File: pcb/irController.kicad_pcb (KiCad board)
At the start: 2 copper layers, 49 x 34 mm, 33 parts, among them J1 B4B-PH-K-S(LF)(SN), P1 ZX62R-B-5P, P2 GPIO_USER, Q1 Q_NMOS, SW2 SKRPACE010, U1 NJM2845, U2 ESP-13-WROOM-02, U3 IRSNS_GP1UXC41QS

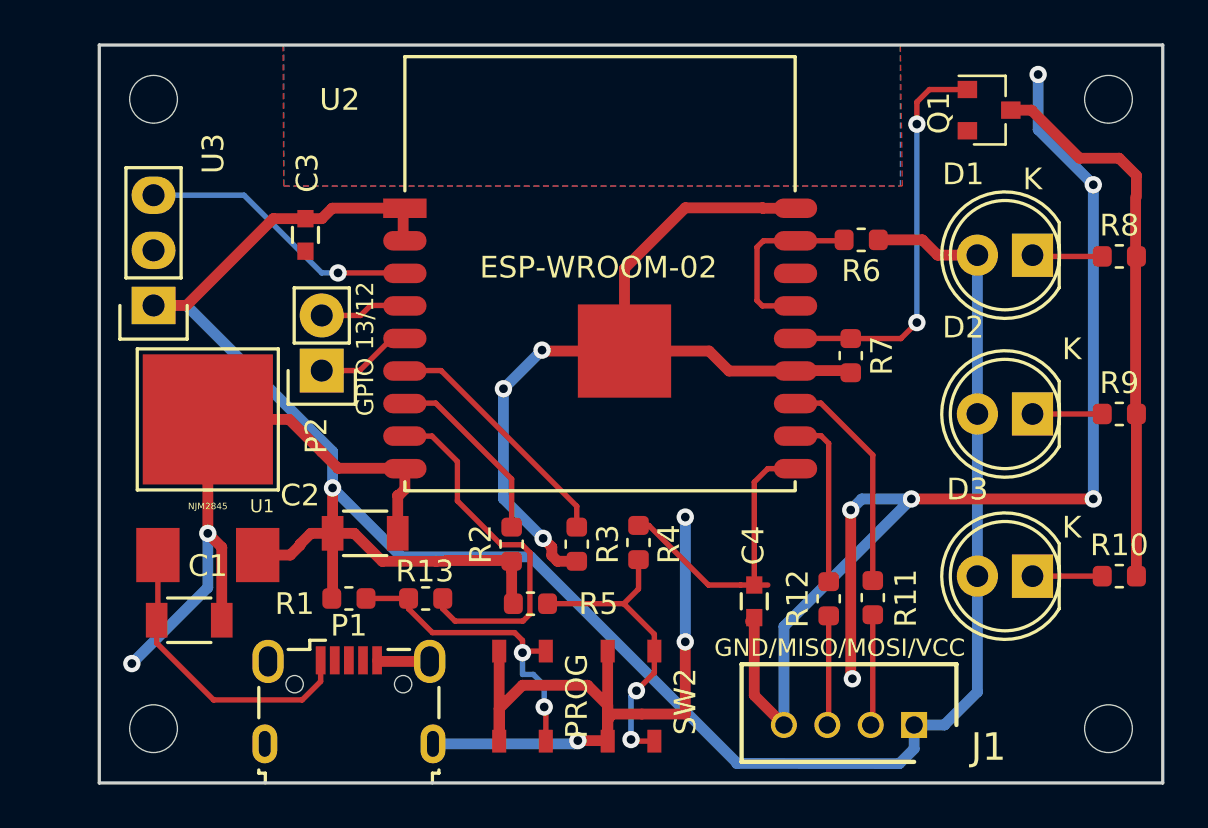
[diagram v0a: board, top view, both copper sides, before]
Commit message: パターン引いた
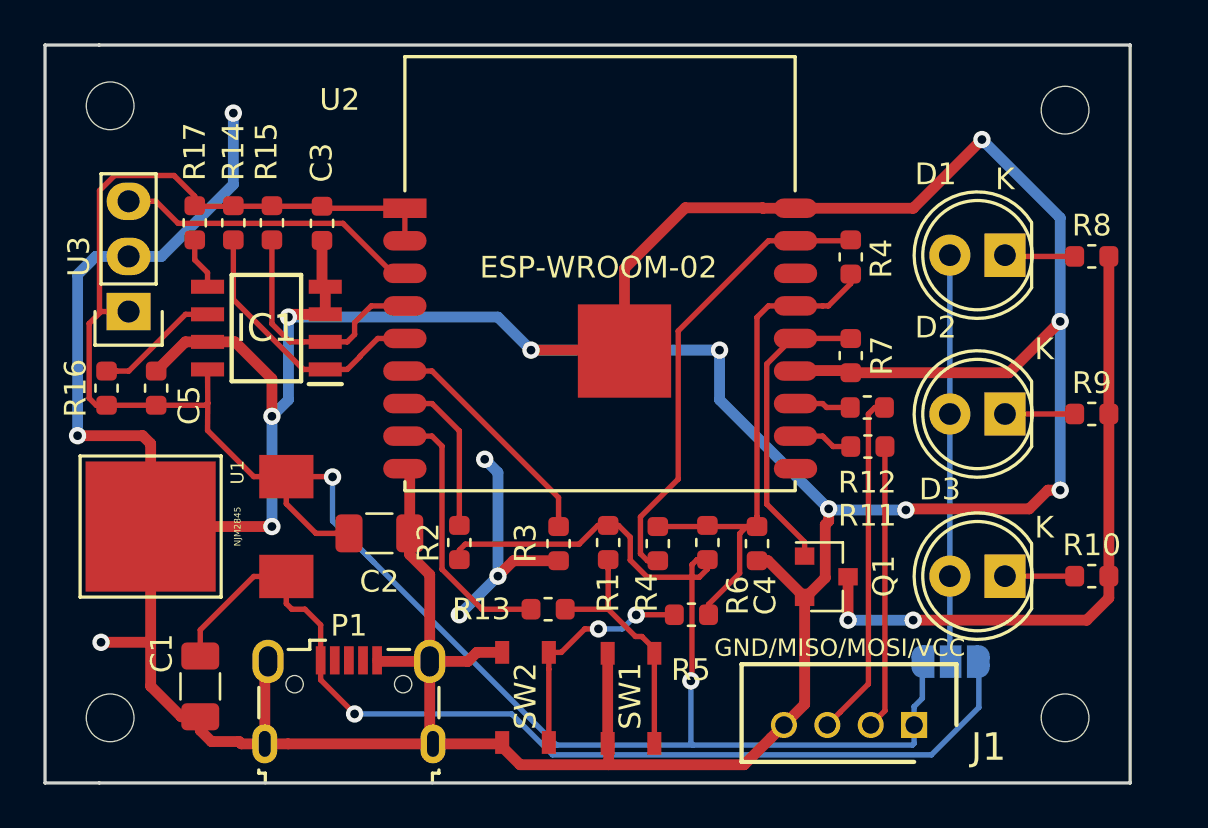
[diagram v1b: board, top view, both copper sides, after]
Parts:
- removed the ? at (134.5, 71.5)
- removed the ? at (134.5, 100.5)
- removed P2: GPIO_USER, Socket_Strips:Socket_Strip_Straight_1x02
- removed PROG: SKRPACE010, OriginalLibSw:SKRPACE010
- added ?: MountingHole_2.2mm_M2, Mounting_Holes:MountingHole_2.2mm_M2, F.Cu at (132.5, 71.8)
- added ?: MountingHole_2.2mm_M2, Mounting_Holes:MountingHole_2.2mm_M2, F.Cu at (132.5, 100.0)
- added C5: 0.1u, Capacitor_SMD:C_0603_1608Metric, F.Cu at (134.6, 84.8)
- added IC1: ADT7410TRZ, SamacSys:SOIC127P600X175-8N, F.Cu at (139.7, 82.0)
- added JP1: SolderJumper_3_Open, Jumper:SolderJumper-3_P1.3mm_Open_RoundedPad1.0x1.5mm_NumberLabels, B.Cu at (171.2, 97.4)
- added R14: 10k, Resistor_SMD:R_0603_1608Metric, F.Cu at (138.2, 77.2)
- added R15: 10k, Resistor_SMD:R_0603_1608Metric, F.Cu at (140.0, 77.2)
- added R16: 10k, Resistor_SMD:R_0603_1608Metric, F.Cu at (132.3, 84.8)
- added R17: 10k, Resistor_SMD:R_0603_1608Metric, F.Cu at (136.4, 77.2)
- added R4: 1k, Resistor_SMD:R_0603_1608Metric, F.Cu at (157.7, 92.0)
- added SW1: SKRPACE010, OriginalLibSw:SKRPACE010, F.Cu at (156.5, 99.1)
- C1, C2: footprint Capacitors_SMD:C_1206 -> Capacitor_SMD:C_1206_3216Metric
- C3: value 0.22u -> 0.1u; footprint Capacitors_SMD:C_0603 -> Capacitor_SMD:C_0603_1608Metric
- C4: footprint Capacitors_SMD:C_0603 -> Capacitor_SMD:C_0603_1608Metric
- R4, R5: value 10k -> 1k
- moved Q1 22.8 mm to (165.5, 93.5)
- moved R4 16.4 mm to (166.6, 78.8)
- moved R6 15.6 mm to (160.0, 91.9), turned to 90 degrees
- moved R1 12.2 mm to (155.4, 91.9), turned to 270 degrees
- moved R12 8.99 mm to (167.4, 85.7), turned to 180 degrees
- moved R5 7.43 mm to (159.3, 95.2), turned to 180 degrees
- moved R11 6.97 mm to (167.4, 87.5), turned to 180 degrees
- moved R13 5.66 mm to (152.7, 95.0), turned to 0 degrees
- moved U1 5.59 mm to (134.4, 91.2), turned to 90 degrees
- moved SW2 4.86 mm to (151.6, 99.1)
- moved C1 3.09 mm to (136.7, 98.6), turned to 270 degrees
- moved C4 2.66 mm to (162.3, 92.0)
- moved R2 2.41 mm to (148.6, 91.9)
- moved ? 2.06 mm to (176.5, 100.0)
- moved ? 2.06 mm to (176.5, 72.0)
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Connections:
- net Net-(C1-Pad1) renamed +5V
- C2 pad 1: Net-(C2-Pad1) -> +3V3
- C3 pad 1: Net-(C2-Pad1) -> +3V3
- D1 pad 2: Net-(C2-Pad1) -> Net-(D1-Pad2)
- D2 pad 2: Net-(C2-Pad1) -> Net-(D1-Pad2)
- D3 pad 2: Net-(C2-Pad1) -> Net-(D1-Pad2)
- J1 pad 1: Net-(C2-Pad1) -> +3V3
- R1 pad 1: Net-(C2-Pad1) -> +3V3
- R2 pad 1: Net-(C2-Pad1) -> +3V3
- R4 pad 1: Net-(R4-Pad1) -> Net-(C4-Pad1)
- R4 pad 2: Net-(C4-Pad1) -> Net-(R4-Pad2)
- R5 pad 1: Net-(C2-Pad1) -> Net-(C4-Pad1)
- R5 pad 2: Net-(R4-Pad1) -> Net-(R5-Pad2)
- R6 pad 1: Net-(C2-Pad1) -> +3V3
- R6 pad 2: Net-(R6-Pad2) -> Net-(C4-Pad1)
- SW2 pad 1: Net-(R4-Pad1) -> Net-(R5-Pad2)
- SW2 pad 3: Net-(R4-Pad1) -> Net-(R5-Pad2)
- U1 pad VO: Net-(C2-Pad1) -> +3V3
- U2 pad 1: Net-(C2-Pad1) -> +3V3
- U2 pad 10: Net-(C4-Pad1) -> Net-(U2-Pad10)
- U2 pad 11: Net-(R12-Pad2) -> Net-(R11-Pad2)
- U2 pad 12: Net-(R11-Pad2) -> Net-(R12-Pad2)
- U2 pad 15: Net-(R6-Pad2) -> Net-(C4-Pad1)
- U2 pad 17: Net-(R6-Pad2) -> Net-(R4-Pad2)
- U2 pad 2: Net-(C2-Pad1) -> +3V3
- U3 pad 1: Net-(C2-Pad1) -> +3V3
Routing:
- net +3V3: track 0.00 -> 111.3 mm, vias 0 -> 2
- net Net-(C2-Pad1): track 109.7 -> 0.00 mm, vias 1 -> 0
- net GND: track 173.7 -> 249.8 mm, vias 14 -> 16
- net +5V: track 14.0 -> 46.7 mm, vias 0 -> 1
- net Net-(R4-Pad2): track 0.00 -> 21.6 mm
- net Net-(D1-Pad2): track 0.00 -> 18.8 mm
- net Net-(R4-Pad1): track 14.2 -> 0.00 mm, vias 2 -> 0
- net Net-(C4-Pad1): track 13.4 -> 24.9 mm
- net Net-(J1-Pad3): track 5.06 -> 16.0 mm
- net Net-(R5-Pad2): track 0.00 -> 10.7 mm, vias 0 -> 2
- net Net-(IC1-Pad1): track 4.37 -> 12.6 mm
- net Net-(J1-Pad2): track 5.12 -> 13.1 mm
- net Net-(R6-Pad2): track 7.88 -> 0.00 mm
- net Net-(IC1-Pad2): track 3.94 -> 11.3 mm
- net Net-(R11-Pad2): track 11.4 -> 4.28 mm
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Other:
- board size 49 x 34 mm -> 50 x 34 mm
- board text added: "IR Remote Controller V1.2"
- board text removed: "GPIO 13/12"
- board text removed: "IR Remote Controller V1.1"
